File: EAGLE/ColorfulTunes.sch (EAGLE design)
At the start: 6 parts, among them U1 0.56_HEX_BACKPACK

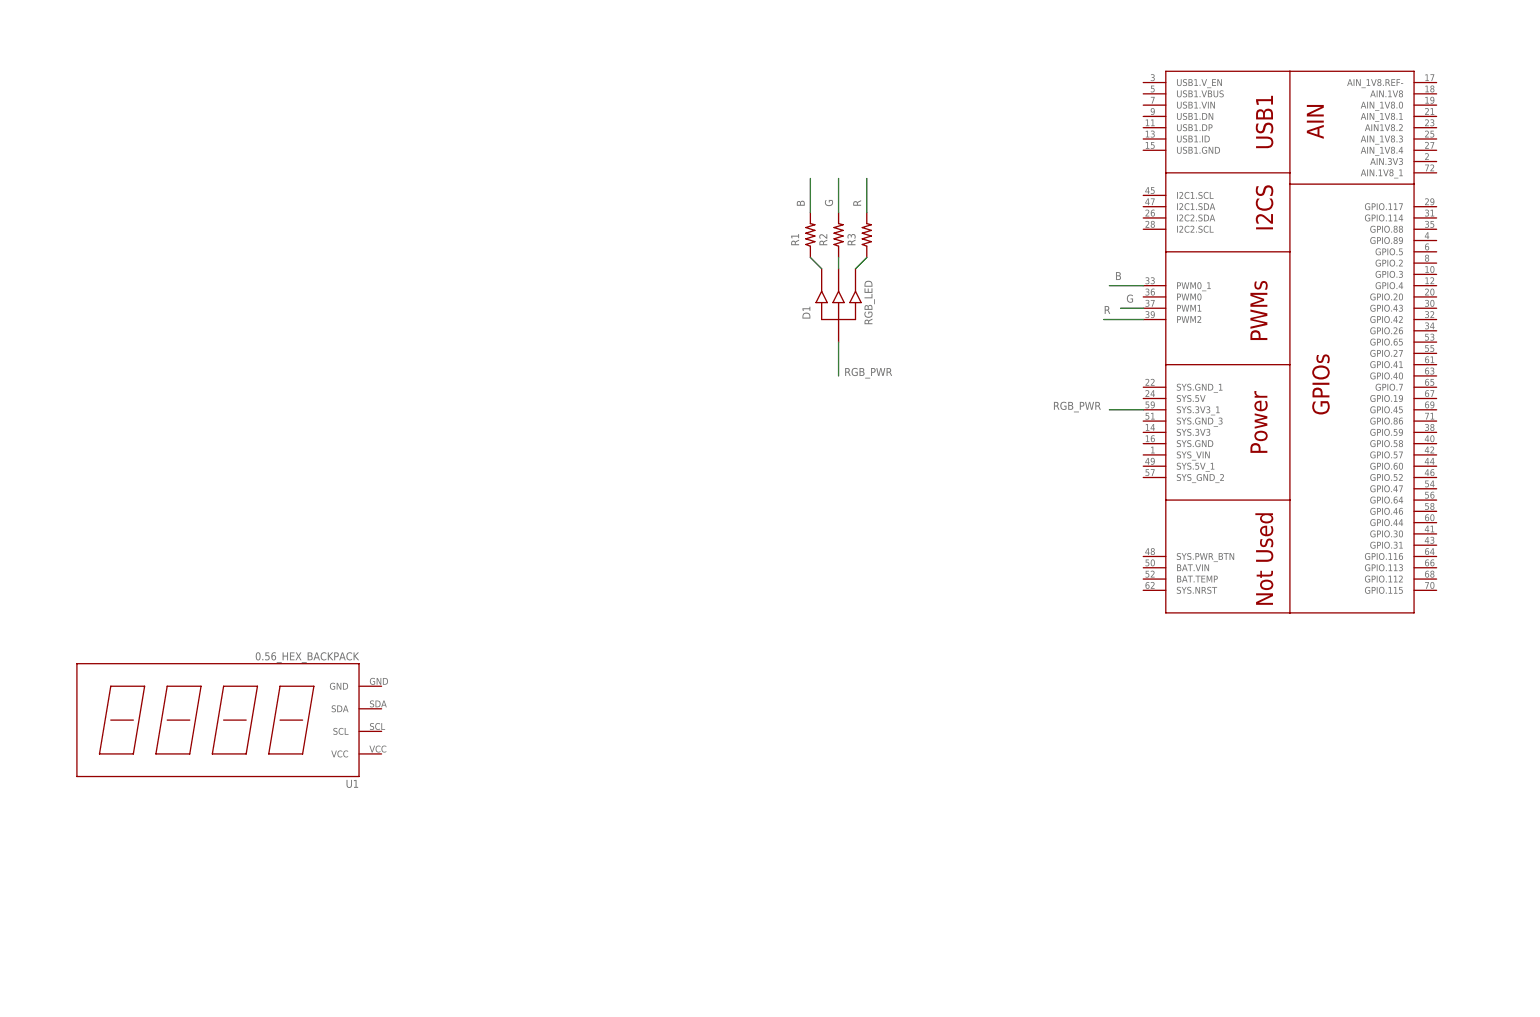
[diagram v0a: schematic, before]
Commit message: Please check this schematic :)
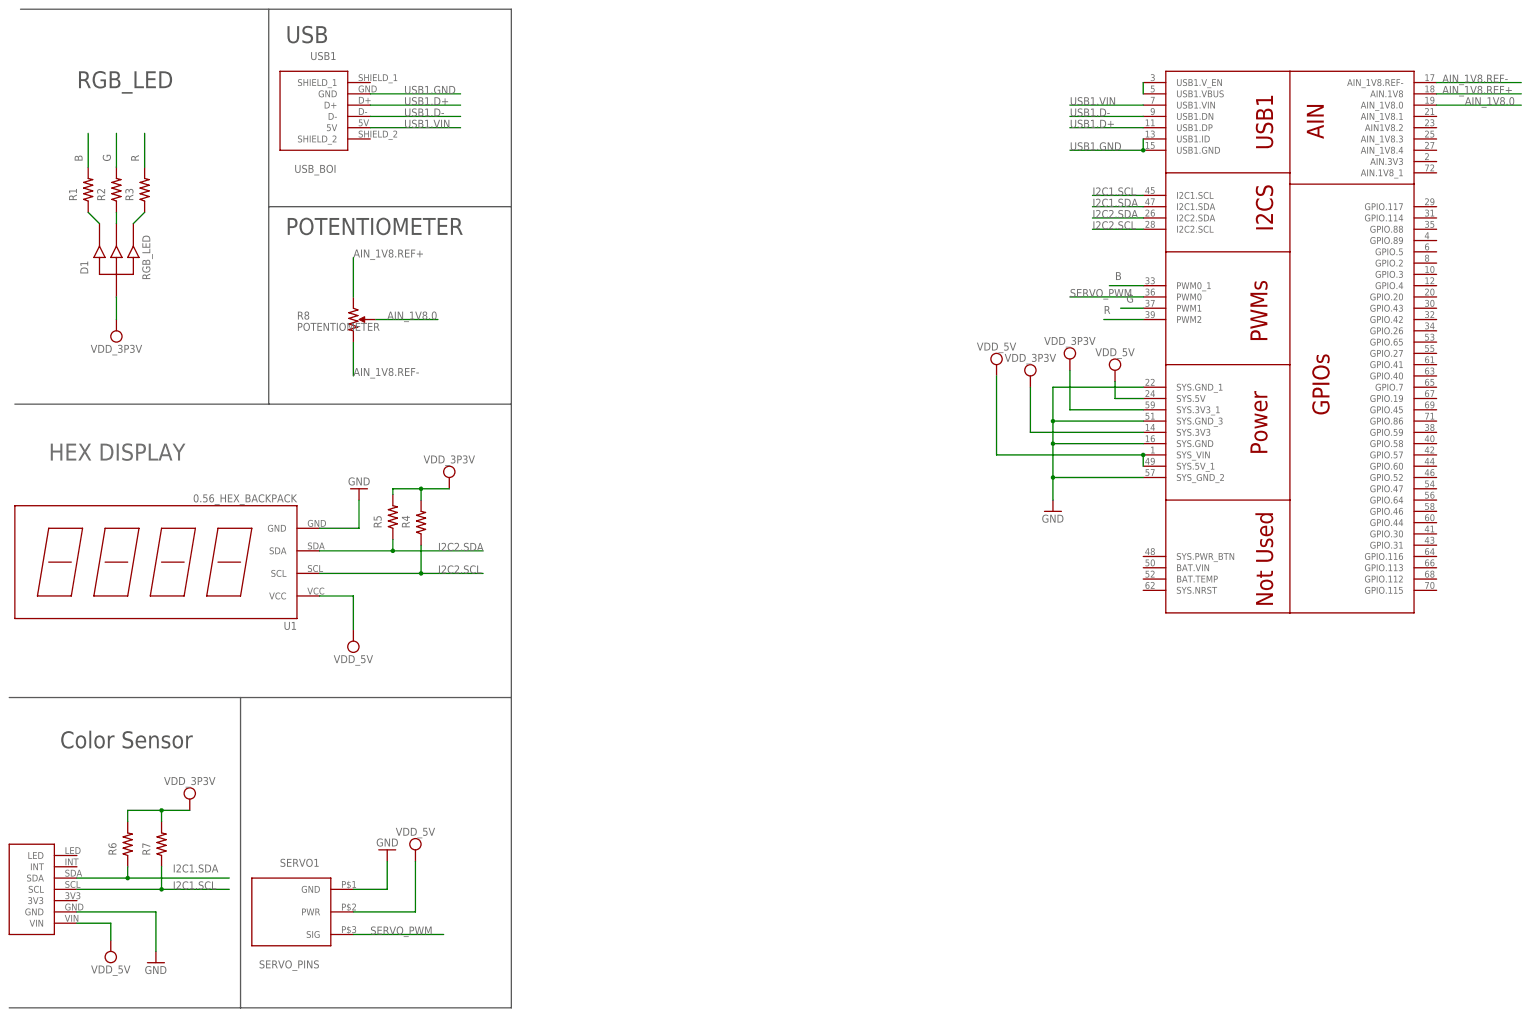
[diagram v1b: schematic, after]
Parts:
- added CS1: COLOR_SENSOR_PINS, ColorfulTunes:COLOR_SENSOR_PINS
- added R4, R5, R6, R7: (no value), ColorfulTunes:R_R0402
- added R8: POTENTIOMETER, ColorfulTunes:POTENTIOMETER
- added SERVO1: SERVO_PINS, ColorfulTunes:SERVO_PINS
- added USB1: USB_BOI, ColorfulTunes:USB_BOI
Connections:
- removed net RGB_PWR: D1.PWR, U$1.SYS.3V3_1
- new net AIN_1V8.0: R8.S, U$1.AIN_1V8.0
- new net AIN_1V8.REF+: R8.CCW, U$1.AIN.1V8
- new net AIN_1V8.REF-: R8.CW, U$1.AIN_1V8.REF-
- new net GND: CS1.GND, SERVO1.GND, U$1.SYS.GND, U$1.SYS.GND_1, U$1.SYS.GND_3, U$1.SYS_GND_2, U1.GND
- new net I2C1.SCL: CS1.SCL, R7.1, U$1.I2C1.SCL
- new net I2C1.SDA: CS1.SDA, R6.1, U$1.I2C1.SDA
- new net I2C2.SCL: R4.1, U$1.I2C2.SCL, U1.SCL
- new net I2C2.SDA: R5.1, U$1.I2C2.SDA, U1.SDA
- new net N$4: U$1.USB1.VBUS, U$1.USB1.V_EN
- new net SERVO_PWM: SERVO1.SIG, U$1.PWM0
- new net USB1.D+: U$1.USB1.DP, USB1.D+
- new net USB1.D-: U$1.USB1.DN, USB1.D-
- new net USB1.GND: U$1.USB1.GND, U$1.USB1.ID, USB1.GND
- new net USB1.VIN: U$1.USB1.VIN, USB1.5V
- new net VDD_3P3V: D1.PWR, R4.2, R5.2, R6.2, R7.2, U$1.SYS.3V3, U$1.SYS.3V3_1
- new net VDD_5V: CS1.VIN, SERVO1.PWR, U$1.SYS.5V, U$1.SYS.5V_1, U$1.SYS_VIN, U1.VCC
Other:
- note added: "Color Sensor"
- note added: "HEX DISPLAY"
- note added: "POTENTIOMETER"
- note added: "RGB_LED"
- note added: "USB"
- moved on the sheet: D1, R1, R2, R3, U1
